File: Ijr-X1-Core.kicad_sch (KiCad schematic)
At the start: 16 parts, among them J1 USB-C_PWR_IN, J2 USB-C_CPU_PROG, J3 USB-C_UART_BRIDGE, U1 RP2040, U2 W25Q16JVSSIQ

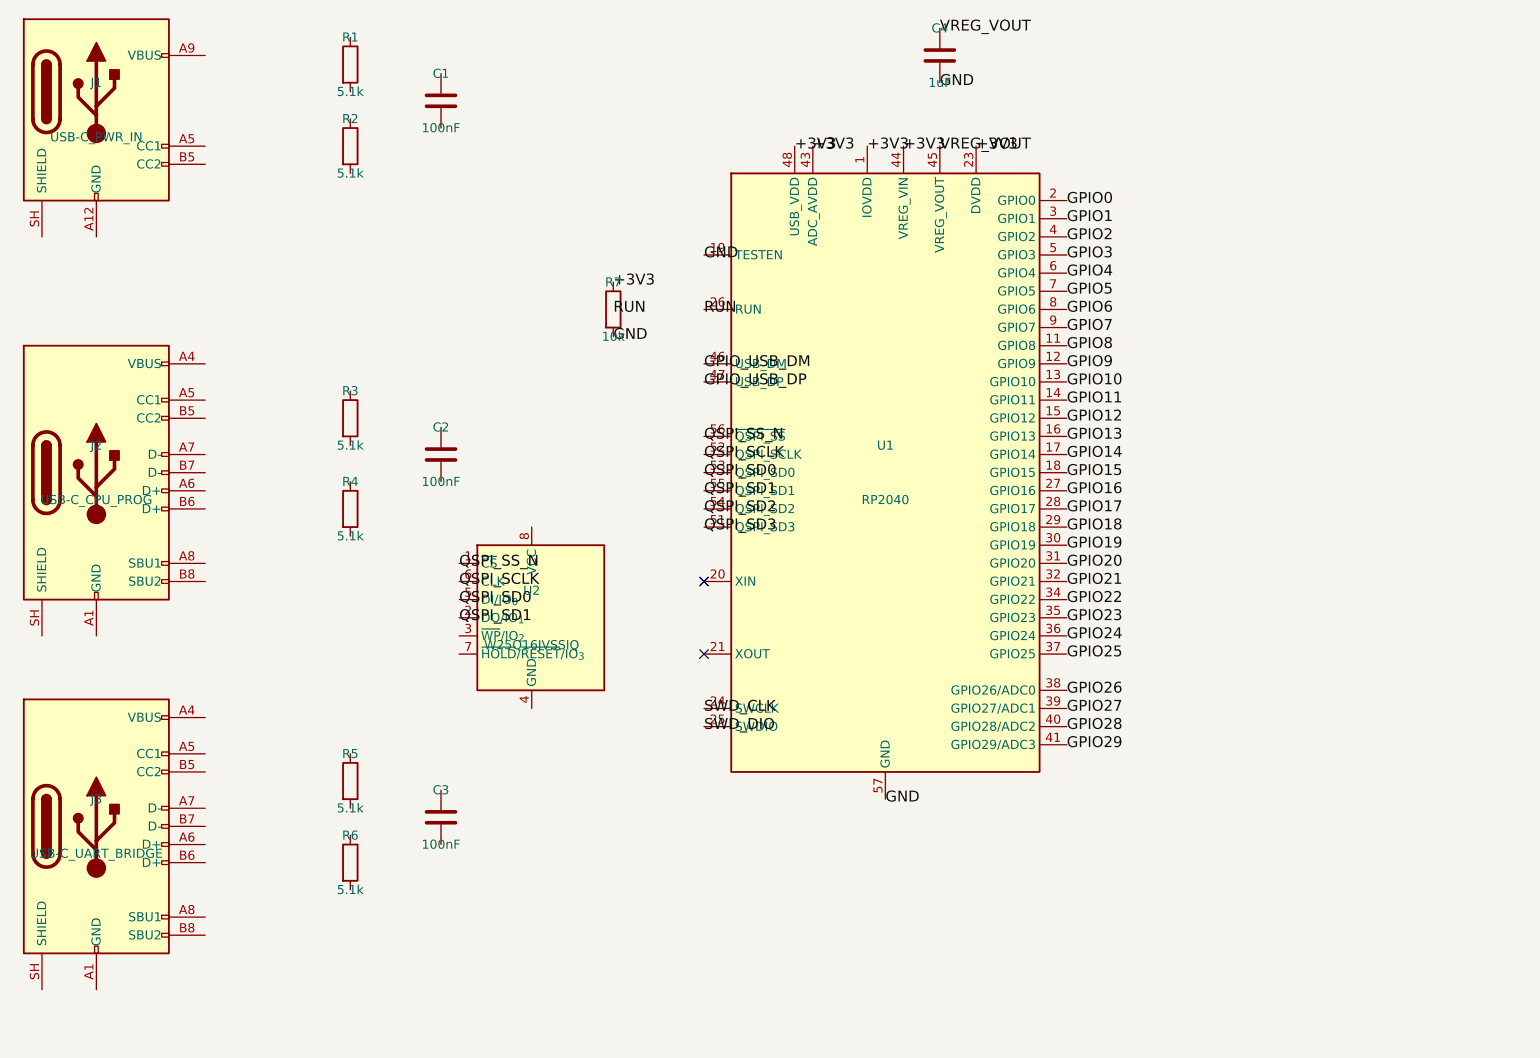
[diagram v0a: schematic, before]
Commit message: Some updates
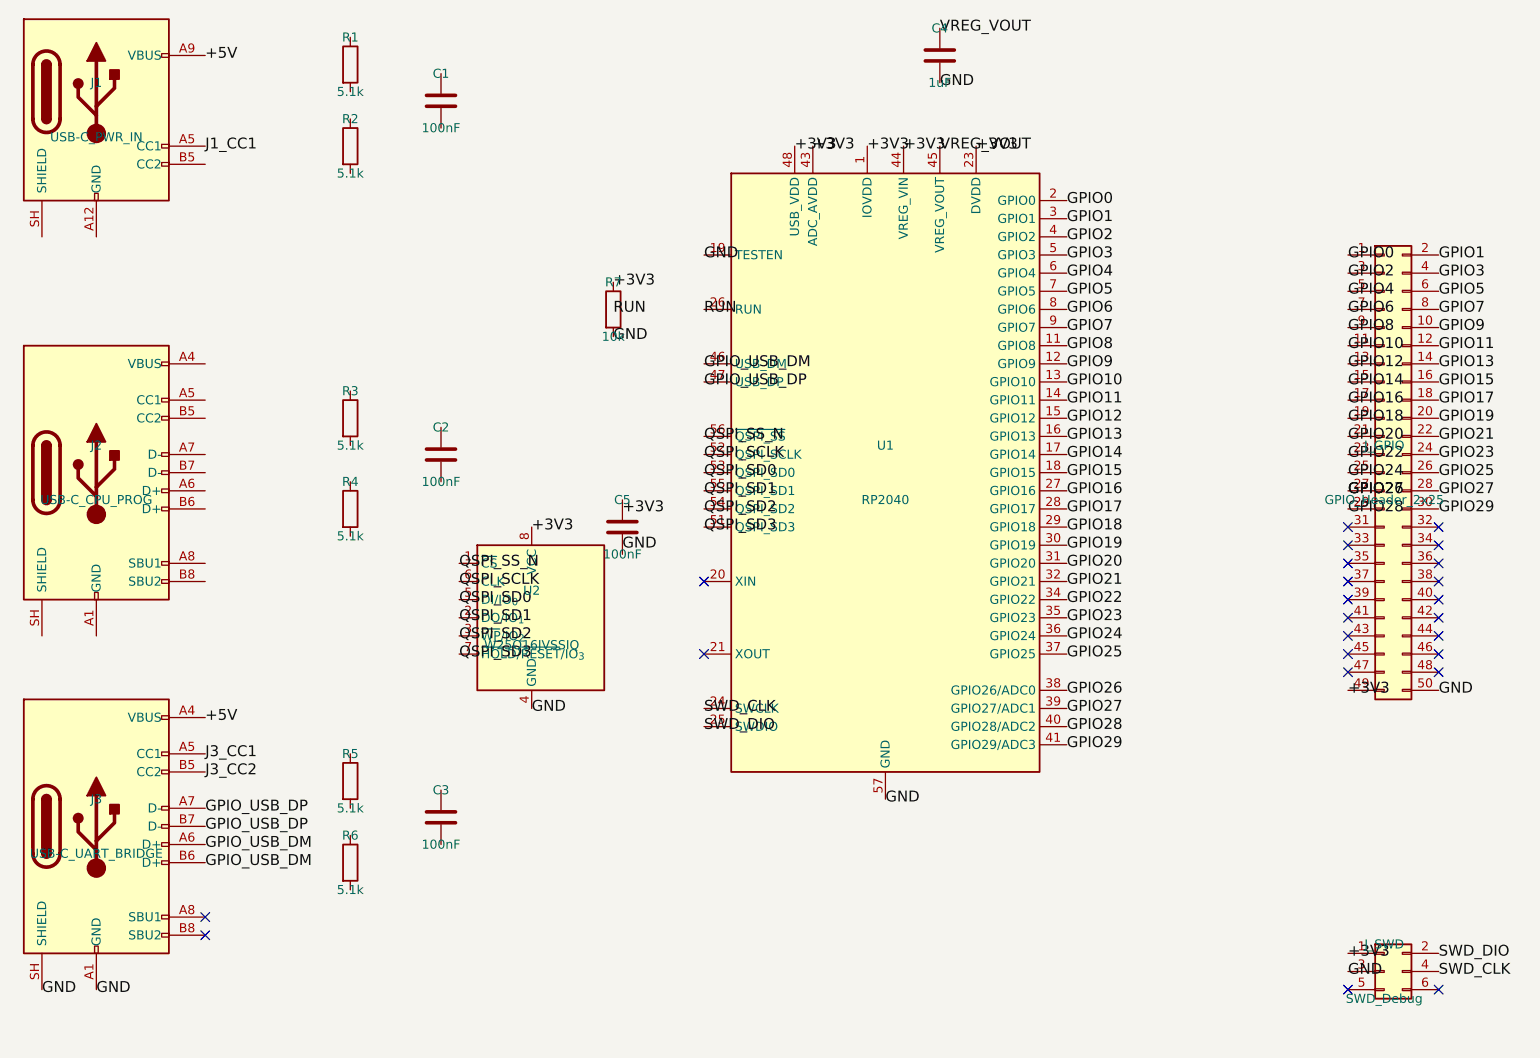
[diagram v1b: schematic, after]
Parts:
- added C5: 100nF, symbol Device:C
- added J_GPIO: GPIO_Header_2x25, symbol Connector_Generic:Conn_02x25_Odd_Even
- added J_SWD: SWD_Debug, symbol Connector_Generic:Conn_02x03_Odd_Even
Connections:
- net GPIO27 is gone; now on net GPIO26: U1.39 (GPIO27/ADC1)
- net +3V3: now also U2.8 (VCC), J_GPIO.49 (Pin_49), J_SWD.1 (Pin_1)
- net GND: now also J3.A1 (GND), J3.A12 (GND), J3.B1 (GND), J3.B12 (GND), J3.SH (SHIELD), U2.4 (GND), J_GPIO.50 (Pin_50), J_SWD.3 (Pin_3)
- net GPIO0: now also J_GPIO.1 (Pin_1)
- net GPIO1: now also J_GPIO.2 (Pin_2)
- net GPIO10: now also J_GPIO.11 (Pin_11)
- net GPIO11: now also J_GPIO.12 (Pin_12)
- net GPIO12: now also J_GPIO.13 (Pin_13)
- net GPIO13: now also J_GPIO.14 (Pin_14)
- net GPIO14: now also J_GPIO.15 (Pin_15)
- net GPIO15: now also J_GPIO.16 (Pin_16)
- net GPIO16: now also J_GPIO.17 (Pin_17)
- net GPIO17: now also J_GPIO.18 (Pin_18)
- net GPIO18: now also J_GPIO.19 (Pin_19)
- net GPIO19: now also J_GPIO.20 (Pin_20)
- net GPIO2: now also J_GPIO.3 (Pin_3)
- net GPIO20: now also J_GPIO.21 (Pin_21)
- net GPIO21: now also J_GPIO.22 (Pin_22)
- net GPIO22: now also J_GPIO.23 (Pin_23)
- net GPIO23: now also J_GPIO.24 (Pin_24)
- net GPIO24: now also J_GPIO.25 (Pin_25)
- net GPIO25: now also J_GPIO.26 (Pin_26)
- net GPIO26: now also J_GPIO.27 (Pin_27), J_GPIO.28 (Pin_28)
- net GPIO28: now also J_GPIO.29 (Pin_29)
- net GPIO29: now also J_GPIO.30 (Pin_30)
- net GPIO3: now also J_GPIO.4 (Pin_4)
- net GPIO4: now also J_GPIO.5 (Pin_5)
- net GPIO5: now also J_GPIO.6 (Pin_6)
- net GPIO6: now also J_GPIO.7 (Pin_7)
- net GPIO7: now also J_GPIO.8 (Pin_8)
- net GPIO8: now also J_GPIO.9 (Pin_9)
- net GPIO9: now also J_GPIO.10 (Pin_10)
- net GPIO_USB_DM: now also J3.A6 (D+), J3.B6 (D+)
- net GPIO_USB_DP: now also J3.A7 (D-), J3.B7 (D-)
- net QSPI_SD2: now also U2.3 (~{WP}/IO_{2})
- net QSPI_SD3: now also U2.7 (~{HOLD}/~{RESET}/IO_{3})
- net SWD_CLK: now also J_SWD.4 (Pin_4)
- net SWD_DIO: now also J_SWD.2 (Pin_2)
- net +5V: now reaches J3.A4 (VBUS), J3.A9 (VBUS), J3.B4 (VBUS), J3.B9 (VBUS)
- net +5V: now also J1.A9 (VBUS), J1.B9 (VBUS)
- net J3_CC1: now reaches J3.A5 (CC1)
- net J3_CC2: now reaches J3.B5 (CC2)
- net J1_CC1: now reaches J1.A5 (CC1)
- no-connect marks 2 -> 24

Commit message: Some updates1
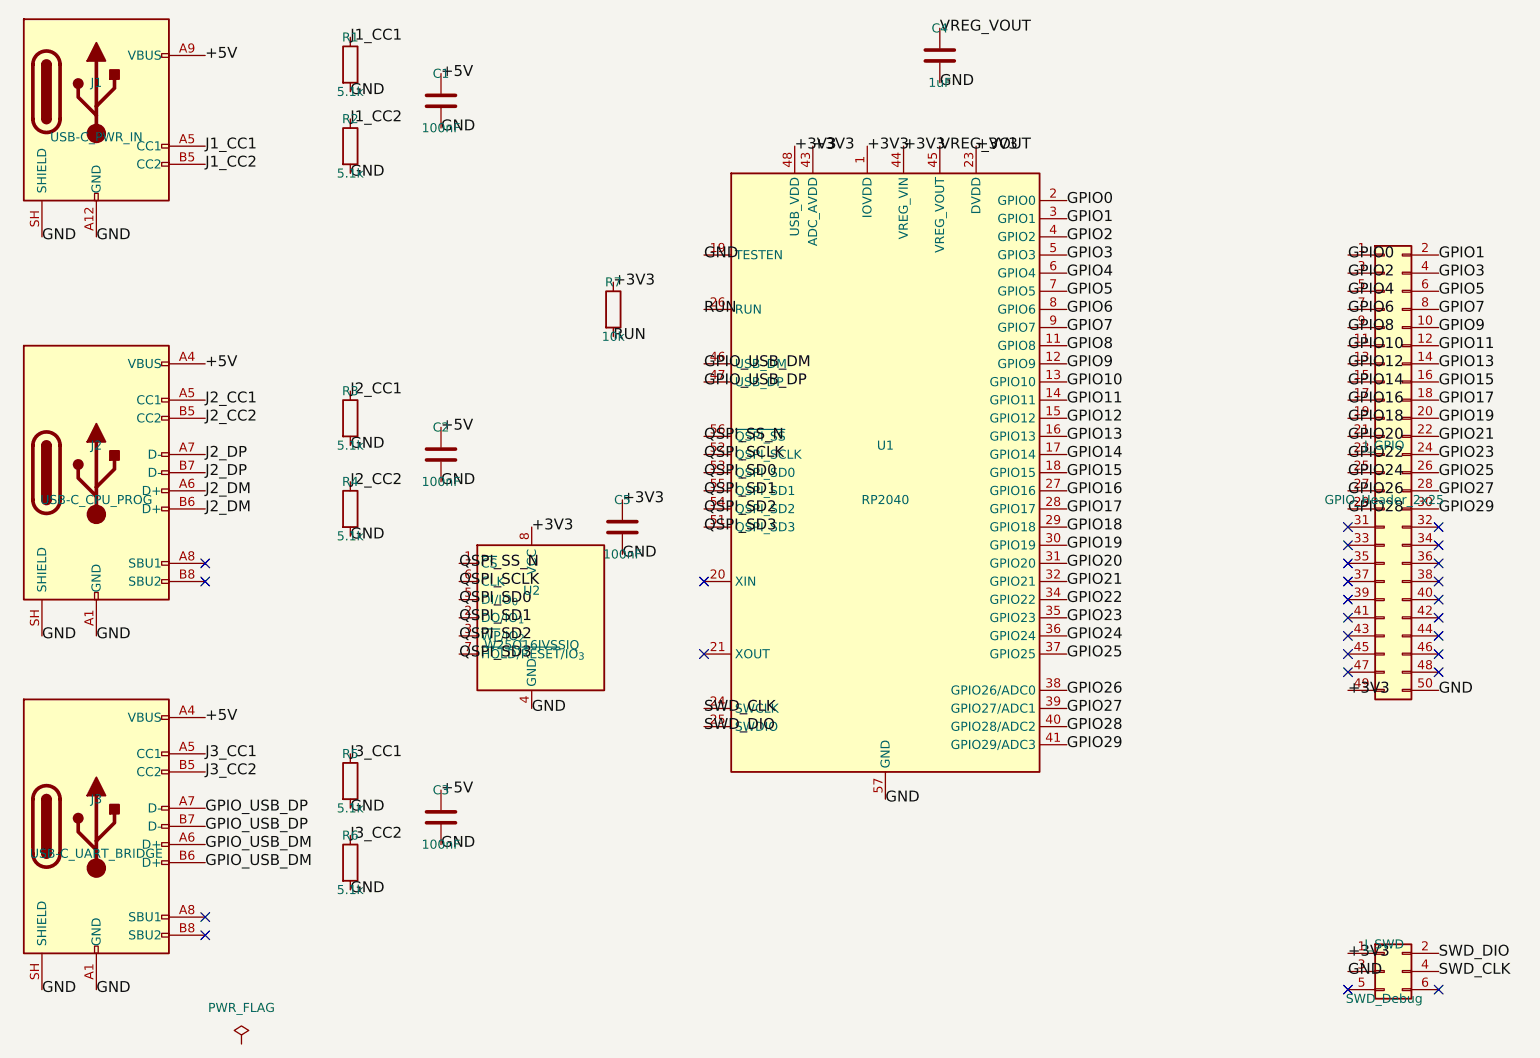
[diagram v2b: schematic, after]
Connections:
- net +3V3: now also C5.1
- net +5V: now also C1.1, C2.1, C3.1, J2.A4 (VBUS), J2.A9 (VBUS), J2.B4 (VBUS), J2.B9 (VBUS)
- net GND: now also C1.2, C2.2, C3.2, C5.2, J1.A12 (GND), J1.B12 (GND), J1.SH (SHIELD), J2.A1 (GND), J2.A12 (GND), J2.B1 (GND), J2.B12 (GND), J2.SH (SHIELD), R1.2, R2.2, R3.2, R4.2, R5.2, R6.2; no longer R7.2
- net GPIO26: no longer J_GPIO.28 (Pin_28), U1.39 (GPIO27/ADC1)
- net J1_CC1: now also R1.1
- net J3_CC1: now also R5.1
- net J3_CC2: now also R6.1
- net RUN: now also R7.2
- net J2_CC2: now reaches R4.1
- net J2_CC2: now also J2.B5 (CC2)
- net J2_CC1: now reaches J2.A5 (CC1)
- net J2_CC1: now also R3.1
- net J2_DM: now reaches J2.A6 (D+)
- net J2_DM: now also J2.B6 (D+)
- net J2_DP: now reaches J2.A7 (D-)
- net J2_DP: now also J2.B7 (D-)
- net J1_CC2: now reaches J1.B5 (CC2)
- net J1_CC2: now also R2.1
- new net GPIO27: J_GPIO.28 (Pin_28), U1.39 (GPIO27/ADC1)
- no-connect marks 24 -> 26
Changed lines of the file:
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@@
-		(effects (font (size 1.524 1.524)))
-	)
-	(label "GND"
-		(at 111.76 71.12 0)
-		(effects (font (size 1.524 1.524)))
-	)
-	(label "RUN"
-		(at 111.76 67.31 0)
 		(effects (font (size 1.524 1.524)))
 	)
@@
 		)
 	)
-	(label "+3V3"
-		(at 113.03 95.25 0)
-		(effects (font (size 1.524 1.524)))
-	)
-	(label "GND"
-		(at 113.03 100.33 0)
-		(effects (font (size 1.524 1.524)))
-	)
 	(symbol
 		(lib_id "Connector_Generic:Conn_02x25_Odd_Even")
@@
 	)
 	(label "GPIO26"
-		(at 214.63 92.71 0)
-		(effects (font (size 1.524 1.524)))
-	)
-	(label "GPIO27"
 		(at 214.63 92.71 0)
 		(effects (font (size 1.524 1.524)))
@@
 		(effects (font (size 1.524 1.524)))
 	)
+	(label "J1_CC2"
+		(at 54.61 46.99 0)
+		(effects (font (size 1.524 1.524)))
+	)
+	(label "GND"
+		(at 39.37 57.15 0)
+		(effects (font (size 1.524 1.524)))
+	)
+	(label "GND"
+		(at 31.75 57.15 0)
+		(effects (font (size 1.524 1.524)))
+	)
+	(label "+5V"
+		(at 54.61 74.93 0)
+		(effects (font (size 1.524 1.524)))
+	)
+	(label "J2_CC1"
+		(at 54.61 80.01 0)
+		(effects (font (size 1.524 1.524)))
+	)
+	(label "J2_CC2"
+		(at 54.61 82.55 0)
+		(effects (font (size 1.524 1.524)))
+	)
+	(label "J2_DP"
+		(at 54.61 87.63 0)
+		(effects (font (size 1.524 1.524)))
+	)
+	(label "J2_DP"
+		(at 54.61 90.17 0)
+		(effects (font (size 1.524 1.524)))
+	)
+	(label "J2_DM"
+		(at 54.61 92.71 0)
+		(effects (font (size 1.524 1.524)))
+	)
+	(label "J2_DM"
+		(at 54.61 95.25 0)
+		(effects (font (size 1.524 1.524)))
+	)
+	(no_connect (at 54.61 102.87))
+	(no_connect (at 54.61 105.41))
+	(label "GND"
+		(at 39.37 113.03 0)
+		(effects (font (size 1.524 1.524)))
+	)
+	(label "GND"
+		(at 31.75 113.03 0)
+		(effects (font (size 1.524 1.524)))
+	)
+	(label "J1_CC1"
+		(at 74.93 29.21 0)
+		(effects (font (size 1.524 1.524)))
+	)
+	(label "GND"
+		(at 74.93 36.83 0)
+		(effects (font (size 1.524 1.524)))
+	)
+	(label "J1_CC2"
+		(at 74.93 40.64 0)
+		(effects (font (size 1.524 1.524)))
+	)
+	(label "GND"
+		(at 74.93 48.26 0)
+		(effects (font (size 1.524 1.524)))
+	)
+	(label "J2_CC1"
+		(at 74.93 78.74 0)
+		(effects (font (size 1.524 1.524)))
+	)
+	(label "GND"
+		(at 74.93 86.36 0)
+		(effects (font (size 1.524 1.524)))
+	)
+	(label "J2_CC2"
+		(at 74.93 91.44 0)
+		(effects (font (size 1.524 1.524)))
+	)
+	(label "GND"
+		(at 74.93 99.06 0)
+		(effects (font (size 1.524 1.524)))
+	)
+	(label "J3_CC1"
+		(at 74.93 129.54 0)
+		(effects (font (size 1.524 1.524)))
+	)
+	(label "GND"
+		(at 74.93 137.16 0)
+		(effects (font (size 1.524 1.524)))
+	)
+	(label "J3_CC2"
+		(at 74.93 140.97 0)
+		(effects (font (size 1.524 1.524)))
+	)
+	(label "GND"
+		(at 74.93 148.59 0)
+		(effects (font (size 1.524 1.524)))
+	)
+	(label "+5V"
+		(at 87.63 34.29 0)
+		(effects (font (size 1.524 1.524)))
+	)
+	(label "GND"
+		(at 87.63 41.91 0)
+		(effects (font (size 1.524 1.524)))
+	)
+	(label "+5V"
+		(at 87.63 83.82 0)
+		(effects (font (size 1.524 1.524)))
+	)
+	(label "GND"
+		(at 87.63 91.44 0)
+		(effects (font (size 1.524 1.524)))
+	)
+	(label "+5V"
+		(at 87.63 134.62 0)
+		(effects (font (size 1.524 1.524)))
+	)
+	(label "GND"
+		(at 87.63 142.24 0)
+		(effects (font (size 1.524 1.524)))
+	)
+	(label "+3V3"
+		(at 113.03 93.98 0)
+		(effects (font (size 1.524 1.524)))
+	)
+	(label "GND"
+		(at 113.03 101.6 0)
+		(effects (font (size 1.524 1.524)))
+	)
+	(label "RUN"
+		(at 111.76 71.12 0)
+		(effects (font (size 1.524 1.524)))
+	)
+	(symbol
+		(lib_id "power:PWR_FLAG")
+		(at 59.69 170.18 0)
+		(unit 1)
+		(exclude_from_sim no)
+		(in_bom yes)
+		(on_board yes)
+		(dnp no)
+		(property "Reference" "#PWR01"
+			(at 59.69 163.83 0)
+			(effects (font (size 1.27 1.27)) (hide yes))
+		)
+		(property "Value" "PWR_FLAG"
+			(at 59.69 165.1 0)
+			(effects (font (size 1.27 1.27)))
+		)
+		(property "Footprint" ""
+			(at 59.69 170.18 0)
+			(effects (font (size 1.27 1.27)) (hide yes))
+		)
+		(property "Datasheet" "~"
+			(at 59.69 170.18 0)
+			(effects (font (size 1.27 1.27)) (hide yes))
+		)
+		(instances
+			(project "Ijr-X1-Core"
+				(path "/0a8e2d86-540d-4bc7-908e-89ff2a8b35b6"
+					(reference "#PWR01") (unit 1)
+				)
+			)
+		)
+	)
 	(sheet_instances
